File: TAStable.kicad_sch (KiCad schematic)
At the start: 20 parts, among them J1 Conn_01x08, J2 ICSP, U1 74HCT1G04, U2 Si5351A-B-GT, U3 74HCT1G04, U4 PIC16LF15313, U5 AZ1117-3.3, U6 74HCT74, Y2 25MHz

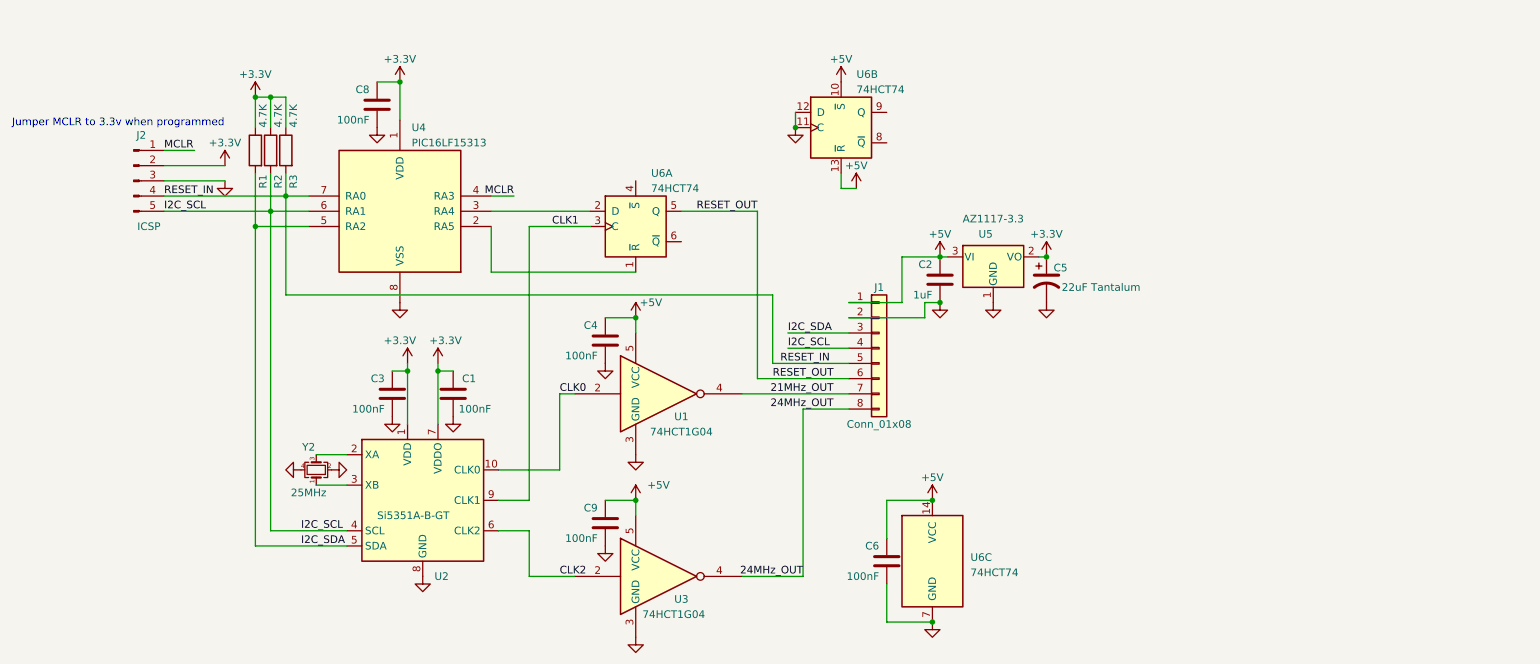
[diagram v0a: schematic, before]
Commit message: andy finally learns FPGA programming
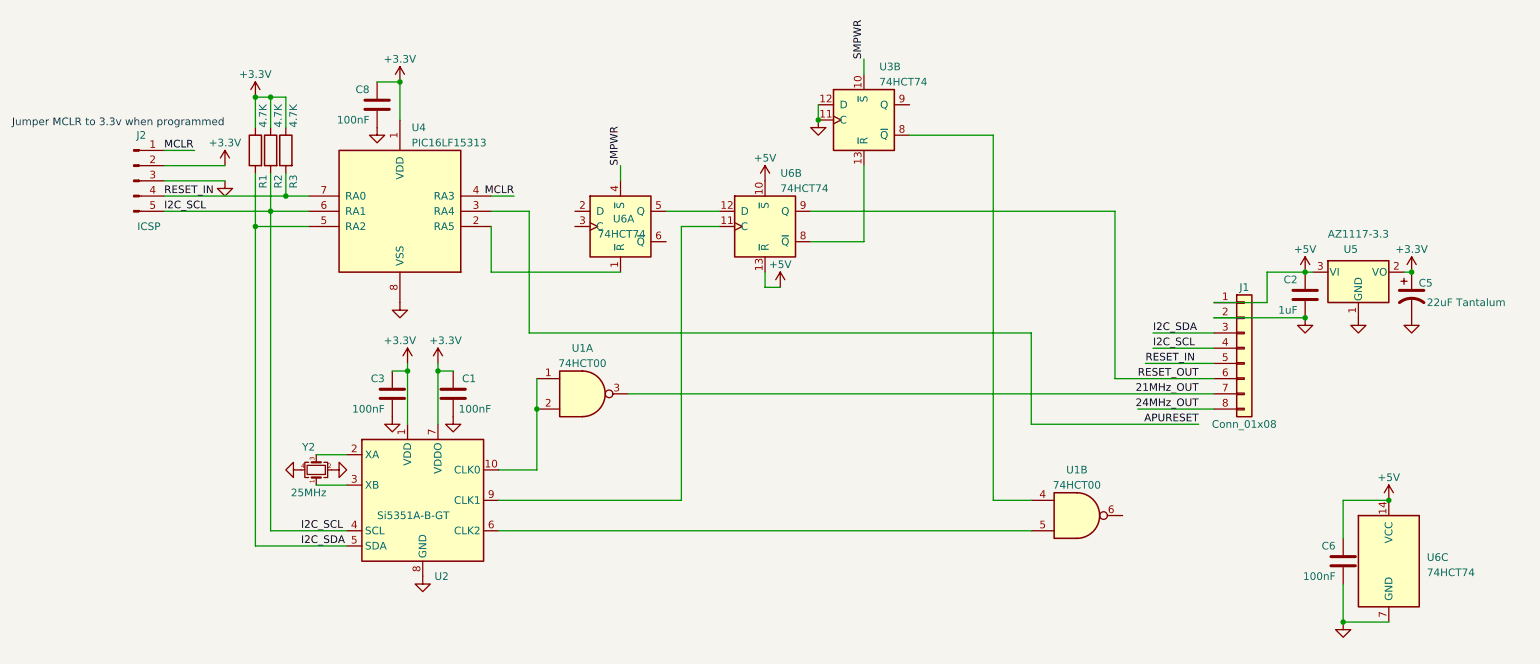
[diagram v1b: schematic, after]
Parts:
- removed C4, C9: 100nF, Capacitor_SMD:C_0603_1608Metric, symbol Device:C
- removed U1, U3: 74HCT1G04, Package_TO_SOT_SMD:SOT-353_SC-70-5, symbol 74xGxx:74AHCT1G04
- added U1: 74HCT00, symbol 74xx:74HCT00
- added U3: 74HCT74, Package_SO:TSSOP-14_4.4x5mm_P0.65mm, symbol 74xx:74HC74
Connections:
- net 21MHz_OUT: now also U1.3
- net GND: now also U3.11 (C), U3.12 (D); no longer U6.11 (C), U6.12 (D)
- net RESET_OUT: now also U6.9 (Q); no longer U6.5 (Q)
- net at U6.8 (~{Q}): now also U3.13 (~{R})
- net at U6.2 (D): no longer U4.3 (RA4)
- net SMPWR: now reaches U6.4 (~{S})
- net SMPWR: now also U3.10 (~{S})
- net CLK0: no longer names the net of U2.10 (CLK0)
- net CLK0: now also U1.1, U1.2
- net CLK1: no longer names the net of U2.9 (CLK1)
- net CLK1: now also U6.11 (C); no longer U6.3 (C)
- net CLK2: no longer names the net of U2.6 (CLK2)
- net CLK2: now also U1.5
- new net: U6.12 (D), U6.5 (Q)
- new net: U1.4, U3.8 (~{Q})
- new net APURESET: U4.3 (RA4)
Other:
- moved on the sheet: C2, C5, C6, J1, U5, U6A, U6B, U6C
